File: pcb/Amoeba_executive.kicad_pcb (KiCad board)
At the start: 2 copper layers, 19 x 22.9 mm, 4 parts, among them J1 Conn_01x04_MountingPin, J2 Conn_01x04_MountingPin, SW1 SW_PUSH_LED

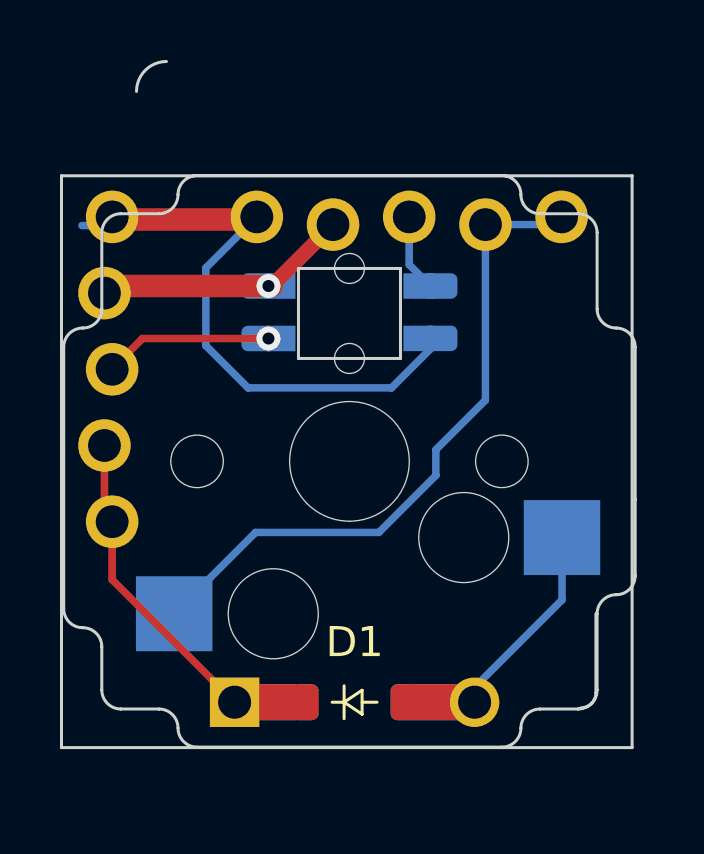
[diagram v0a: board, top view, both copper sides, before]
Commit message: First draft complete
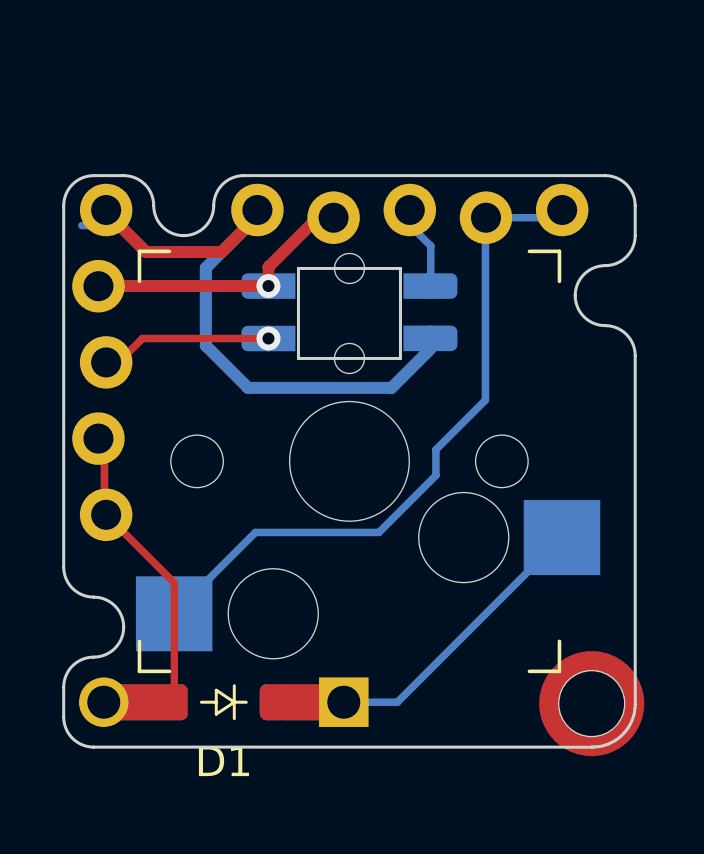
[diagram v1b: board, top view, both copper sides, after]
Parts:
- added REF**: Amoeba_MountingHole_2.2mm_M2_DIN965_Pad_TopOnly, ergodonk_kicad_library:Amoeba_MountingHole_2.2mm_M2_DIN965_Pad_TopOnly, F.Cu at (189.8, 93.5)
- added REF**: 2.54 gird, ergodonk_kicad_library:2.54 gird, F.Cu at (178.7, 86.5)
- moved D1 4.36 mm to (177.5, 93.4), turned to 180 degrees
- moved J2 0.30 mm to (173.5, 82.1)
- moved J1 0.23 mm to (183.7, 77.1)
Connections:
- D1 pad 1: /Row -> Net-(D1-K)
- D1 pad 2: Net-(D1-A) -> /Row
- SW1 pad 5: Net-(D1-A) -> Net-(D1-K)
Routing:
- net Net-(D1-K): track 0.00 -> 9.55 mm
- net Net-(D1-A): track 6.70 -> 0.00 mm
- net /Row: track 10.9 -> 9.83 mm
- net GND: track 19.7 -> 20.6 mm
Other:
- board size 19 x 22.9 mm -> 19.1 x 19 mm
